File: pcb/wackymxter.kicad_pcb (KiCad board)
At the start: 2 copper layers, 181 x 128.6 mm, 72 parts, among them J1 OLED_128x32, SW1 Switch, U2 Raspberry_Pi_Pico, U3 TRRS

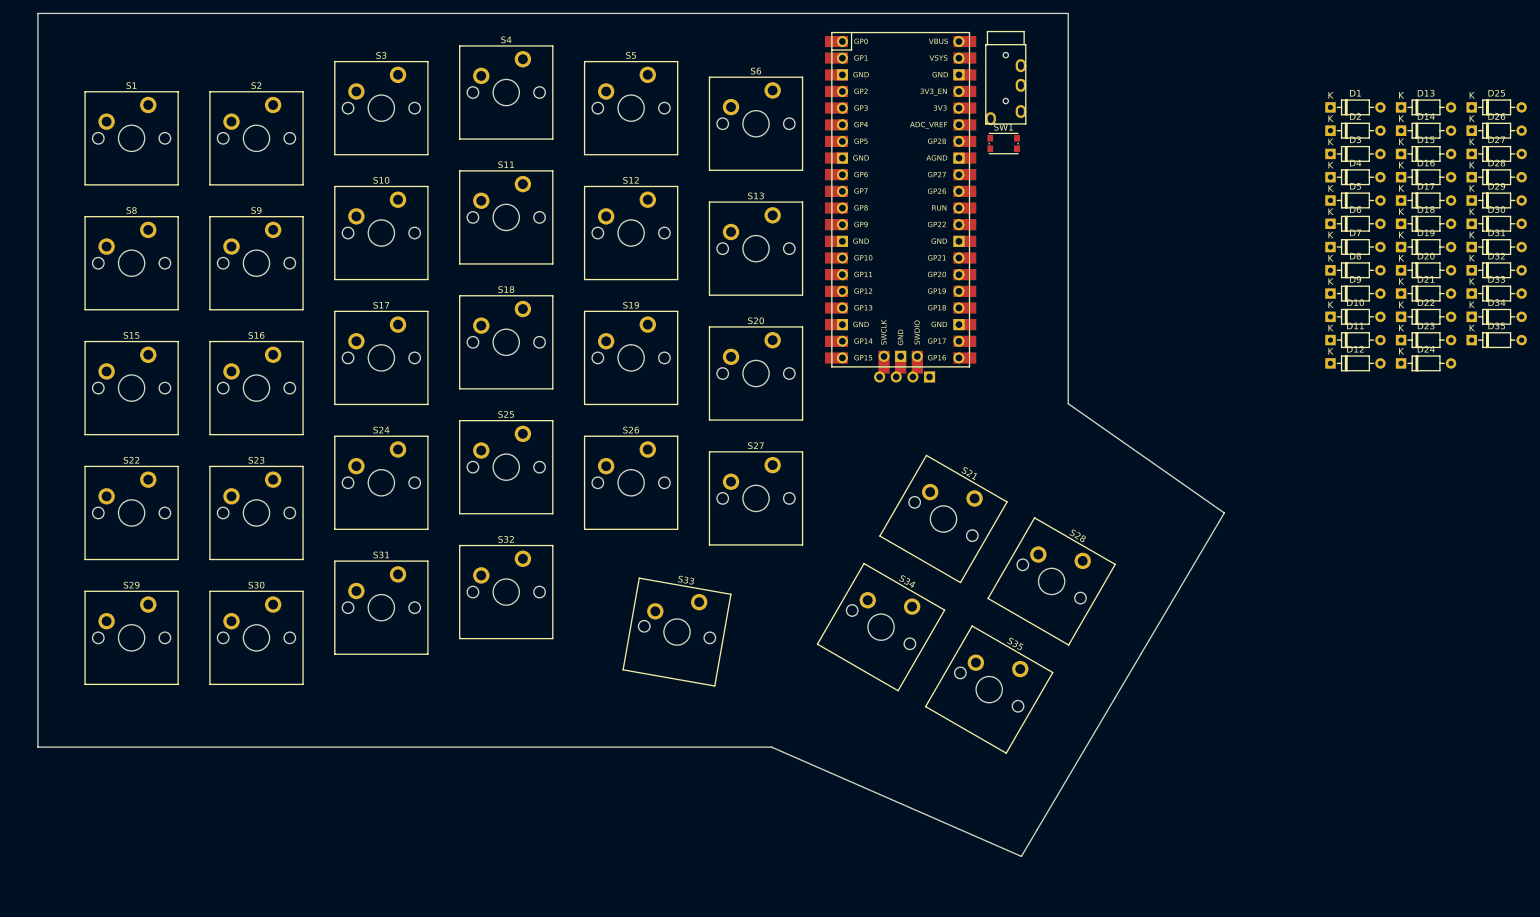
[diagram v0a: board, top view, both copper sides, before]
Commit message: [KiCAD] V0.1: fully connected pcb
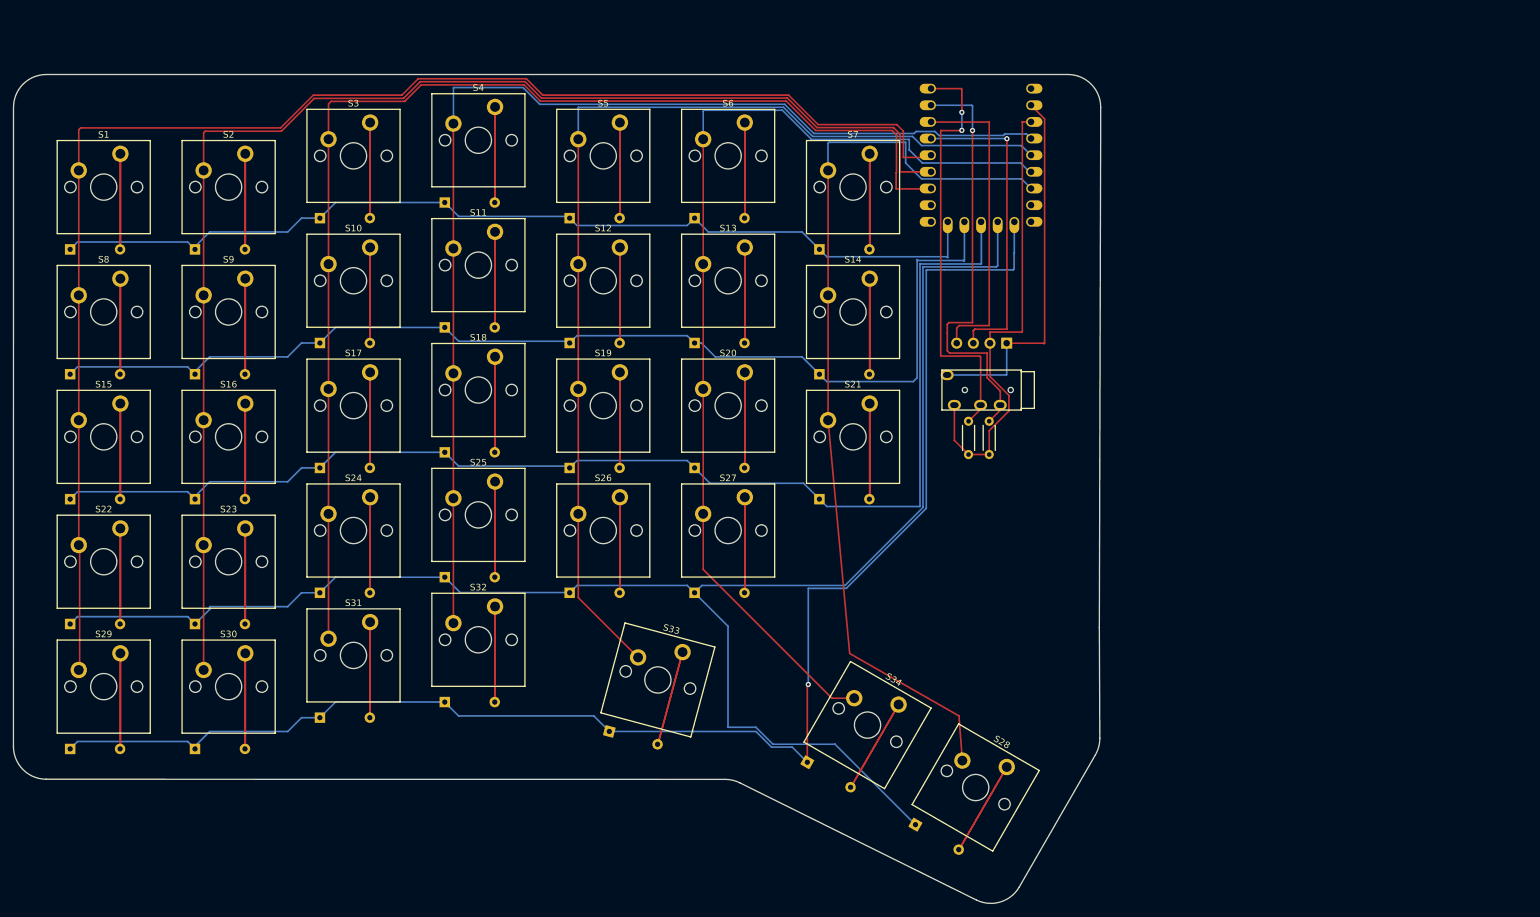
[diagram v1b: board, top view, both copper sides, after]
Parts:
- removed D35: Diode, ScottoKeebs_Components:Diode_DO-35
- removed S35: Keyswitch, ScottoKeebs_MX:MX_PCB_1.00u
- removed SW1: Switch, Button_Switch_SMD:SW_Push_1P1T_NO_CK_KMR2
- removed U2: Raspberry_Pi_Pico, ScottoKeebs_MCU:Raspberry_Pi_Pico
- added R1: Resistor, Resistor_THT:R_Axial_DIN0204_L3.6mm_D1.6mm_P5.08mm_Horizontal, F.Cu at (176.0, 82.5)
- added R2: Resistor, Resistor_THT:R_Axial_DIN0204_L3.6mm_D1.6mm_P5.08mm_Horizontal, F.Cu at (179.1, 82.5)
- added S14: Keyswitch, ScottoKeebs_MX:MX_PCB_1.00u, F.Cu at (158.3, 60.7)
- added S7: Keyswitch, ScottoKeebs_MX:MX_PCB_1.00u, F.Cu at (158.3, 41.7)
- added U1: RP2040_Zero, ScottoKeebs_MCU:RP2040_Zero, B.Cu at (177.9, 36.8)
- D1, D10, D11, D12, D13, D14, D15, D16, D17, D18, D19, D2, D20, D21, D22, D23, D24, D25, D26, D27, D28, D29, D3, D30, D31, D32, D33, D34, D4, D5, D6, D7, D8, D9: moved to B.Cu
- S33: footprint ScottoKeebs_MX:MX_PCB_1.50u -> ScottoKeebs_MX:MX_PCB_1.00u
- moved D29 229.6 mm to (38.9, 127.4)
- moved D30 210.6 mm to (58.0, 127.4)
- moved D15 209.7 mm to (38.9, 89.3)
- moved D22 208.4 mm to (38.9, 108.3)
- moved D1 193.5 mm to (38.9, 51.2)
- moved D8 192.9 mm to (38.9, 70.2)
- moved D16 190.4 mm to (58.0, 89.3)
- moved D31 189.8 mm to (77.0, 122.6)
- moved D23 189.0 mm to (58.0, 108.3)
- moved D2 174.1 mm to (58.0, 51.2)
- moved D9 173.6 mm to (58.0, 70.2)
- moved D25 172.3 mm to (96.1, 101.2)
- moved D32 169.9 mm to (96.1, 120.2)
- moved D17 169.9 mm to (77.0, 84.5)
- moved D24 168.6 mm to (77.0, 103.6)
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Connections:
- U3 pad 2: TX0 -> VCC
- U3 pad 3: RX0 -> TX0
- U3 pad 4: VCC -> RX0
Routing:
- net row3: track 0.00 -> 253.8 mm
- net row4: track 0.00 -> 227.0 mm, vias 0 -> 1
- net col0: track 0.00 -> 223.2 mm
- net col1: track 0.00 -> 205.2 mm
- net row2: track 0.00 -> 191.0 mm
- net col2: track 0.00 -> 186.2 mm
- net col3: track 0.00 -> 173.4 mm
- net row1: track 0.00 -> 169.2 mm
- net col4: track 0.00 -> 159.8 mm
- net col5: track 0.00 -> 156.0 mm
- net row0: track 0.00 -> 147.9 mm
- net col6: track 0.00 -> 139.8 mm
- net VCC: track 0.00 -> 71.0 mm
- net RX0: track 0.00 -> 65.6 mm, vias 0 -> 1
- net TX0: track 0.00 -> 65.3 mm, vias 0 -> 2
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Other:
- board size 181 x 128.6 mm -> 165.9 x 126.4 mm
